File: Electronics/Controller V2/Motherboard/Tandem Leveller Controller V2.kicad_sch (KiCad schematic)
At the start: 0 parts

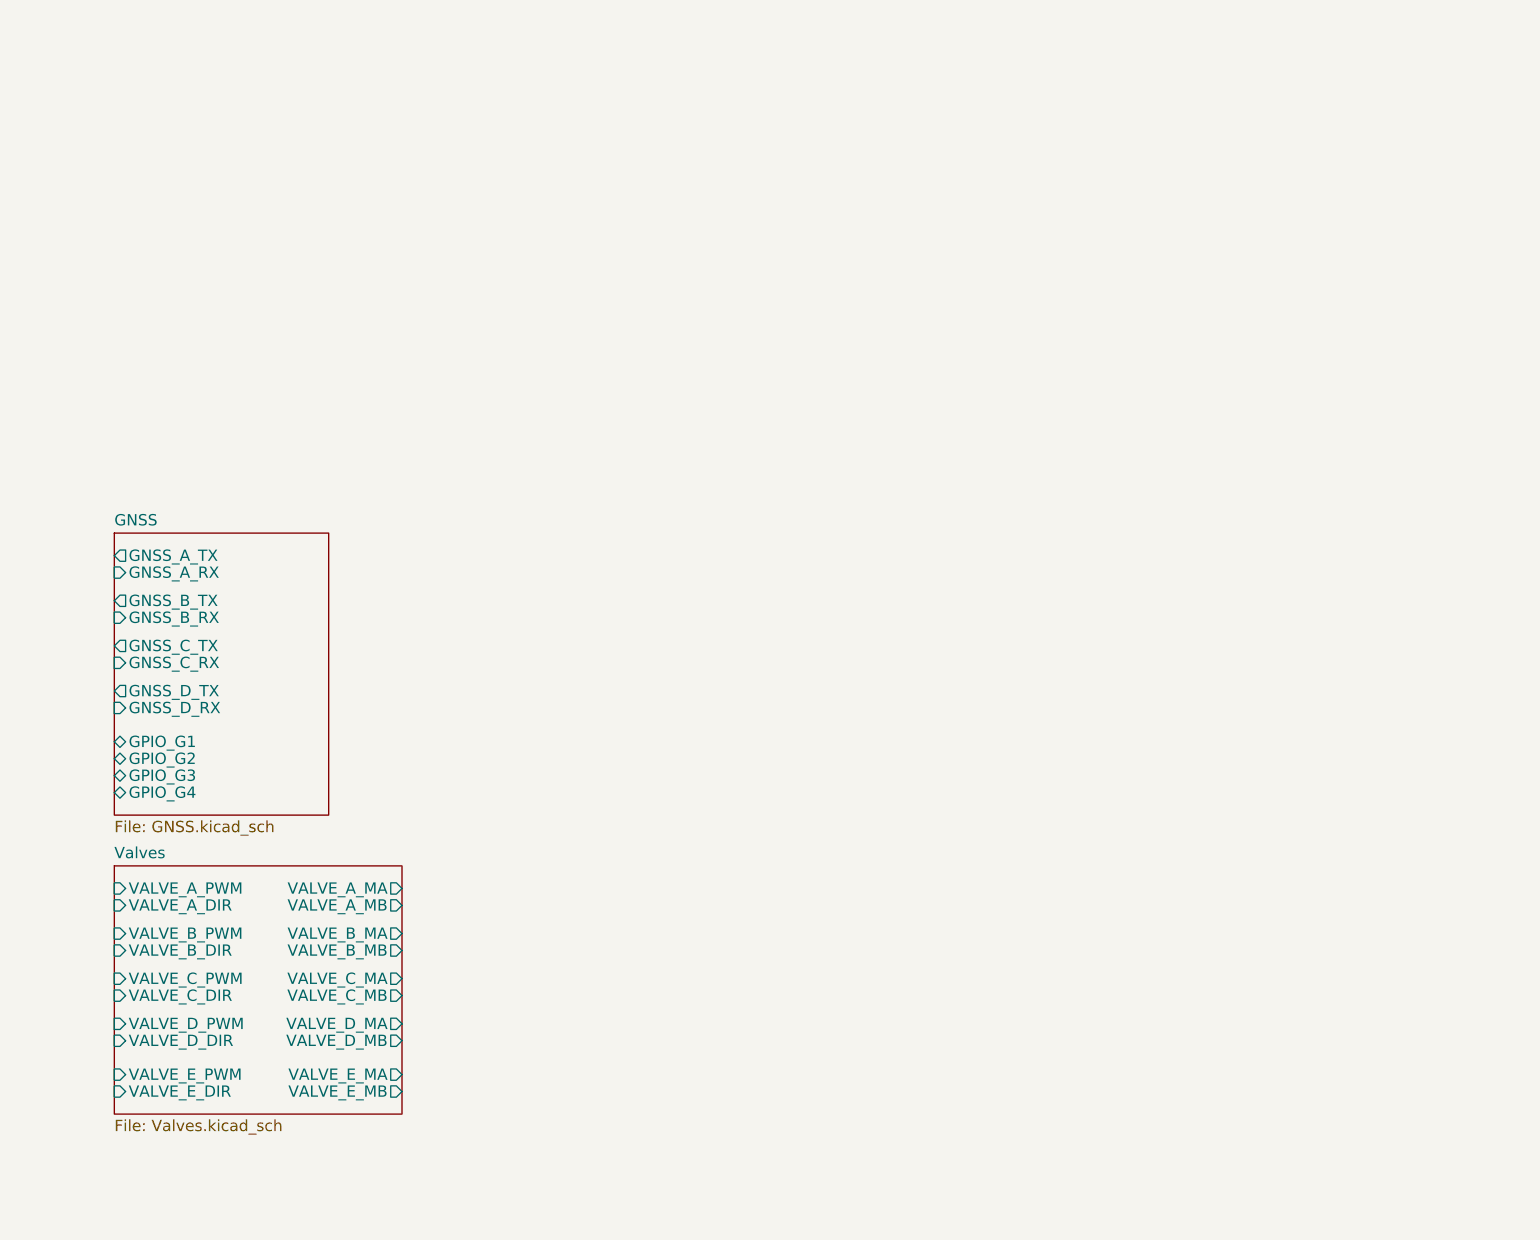
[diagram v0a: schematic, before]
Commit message: WIP
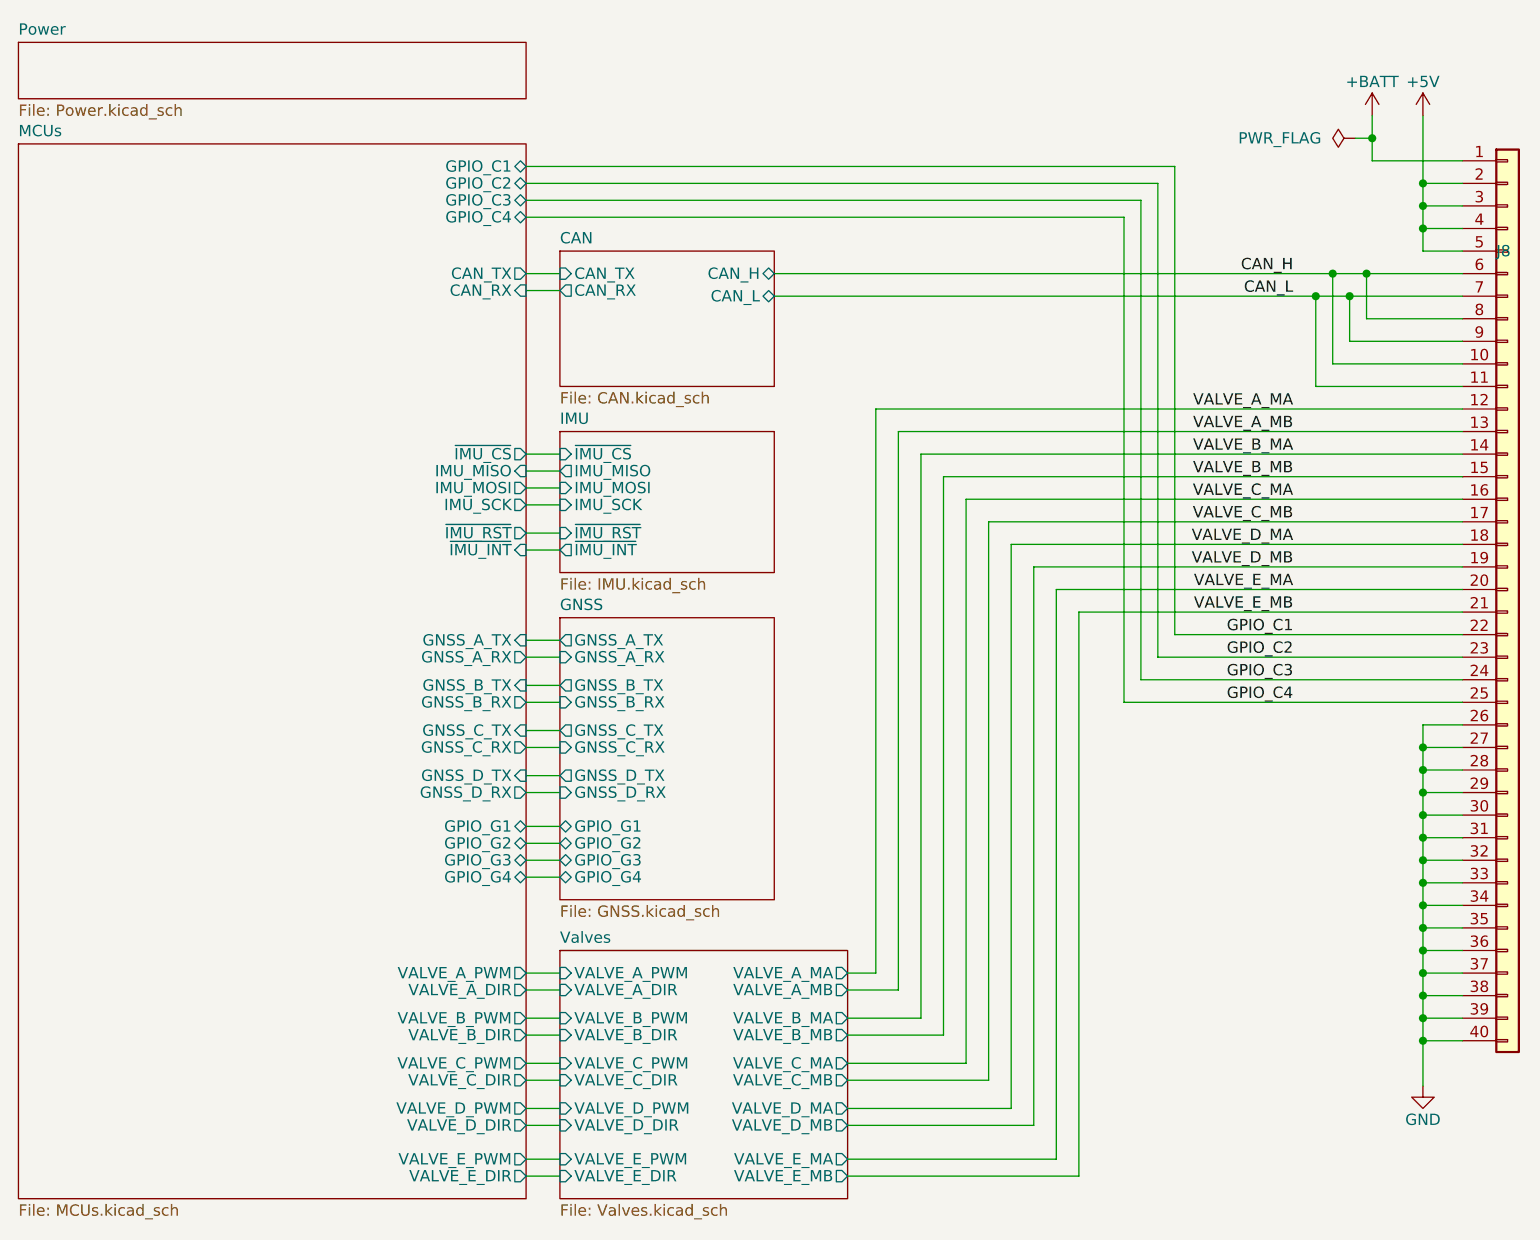
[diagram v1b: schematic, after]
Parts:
- added J8: Conn_01x30, symbol Connector_Generic:Conn_01x40
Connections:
- new net +5V: J8.2 (Pin_2), J8.3 (Pin_3), J8.4 (Pin_4), J8.5 (Pin_5)
- new net +BATT: J8.1 (Pin_1)
- new net CAN_H: J8.10 (Pin_10), J8.6 (Pin_6), J8.8 (Pin_8)
- new net CAN_L: J8.11 (Pin_11), J8.7 (Pin_7), J8.9 (Pin_9)
- new net GND: J8.26 (Pin_26), J8.27 (Pin_27), J8.28 (Pin_28), J8.29 (Pin_29), J8.30 (Pin_30), J8.31 (Pin_31), J8.32 (Pin_32), J8.33 (Pin_33), J8.34 (Pin_34), J8.35 (Pin_35), J8.36 (Pin_36), J8.37 (Pin_37), J8.38 (Pin_38), J8.39 (Pin_39), J8.40 (Pin_40)
- new net GPIO_C1: J8.22 (Pin_22)
- new net GPIO_C2: J8.23 (Pin_23)
- new net GPIO_C3: J8.24 (Pin_24)
- new net GPIO_C4: J8.25 (Pin_25)
- new net VALVE_A_MA: J8.12 (Pin_12)
- new net VALVE_A_MB: J8.13 (Pin_13)
- new net VALVE_B_MA: J8.14 (Pin_14)
- new net VALVE_B_MB: J8.15 (Pin_15)
- new net VALVE_C_MA: J8.16 (Pin_16)
- new net VALVE_C_MB: J8.17 (Pin_17)
- new net VALVE_D_MA: J8.18 (Pin_18)
- new net VALVE_D_MB: J8.19 (Pin_19)
- new net VALVE_E_MA: J8.20 (Pin_20)
- new net VALVE_E_MB: J8.21 (Pin_21)
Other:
- added sheet CAN (CAN.kicad_sch)
- added sheet IMU (IMU.kicad_sch)
- added sheet MCUs (MCUs.kicad_sch)
- added sheet Power (Power.kicad_sch)
